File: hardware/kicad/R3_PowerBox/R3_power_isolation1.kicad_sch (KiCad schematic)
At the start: 13 parts, among them U3 RS3E-0505S/H3

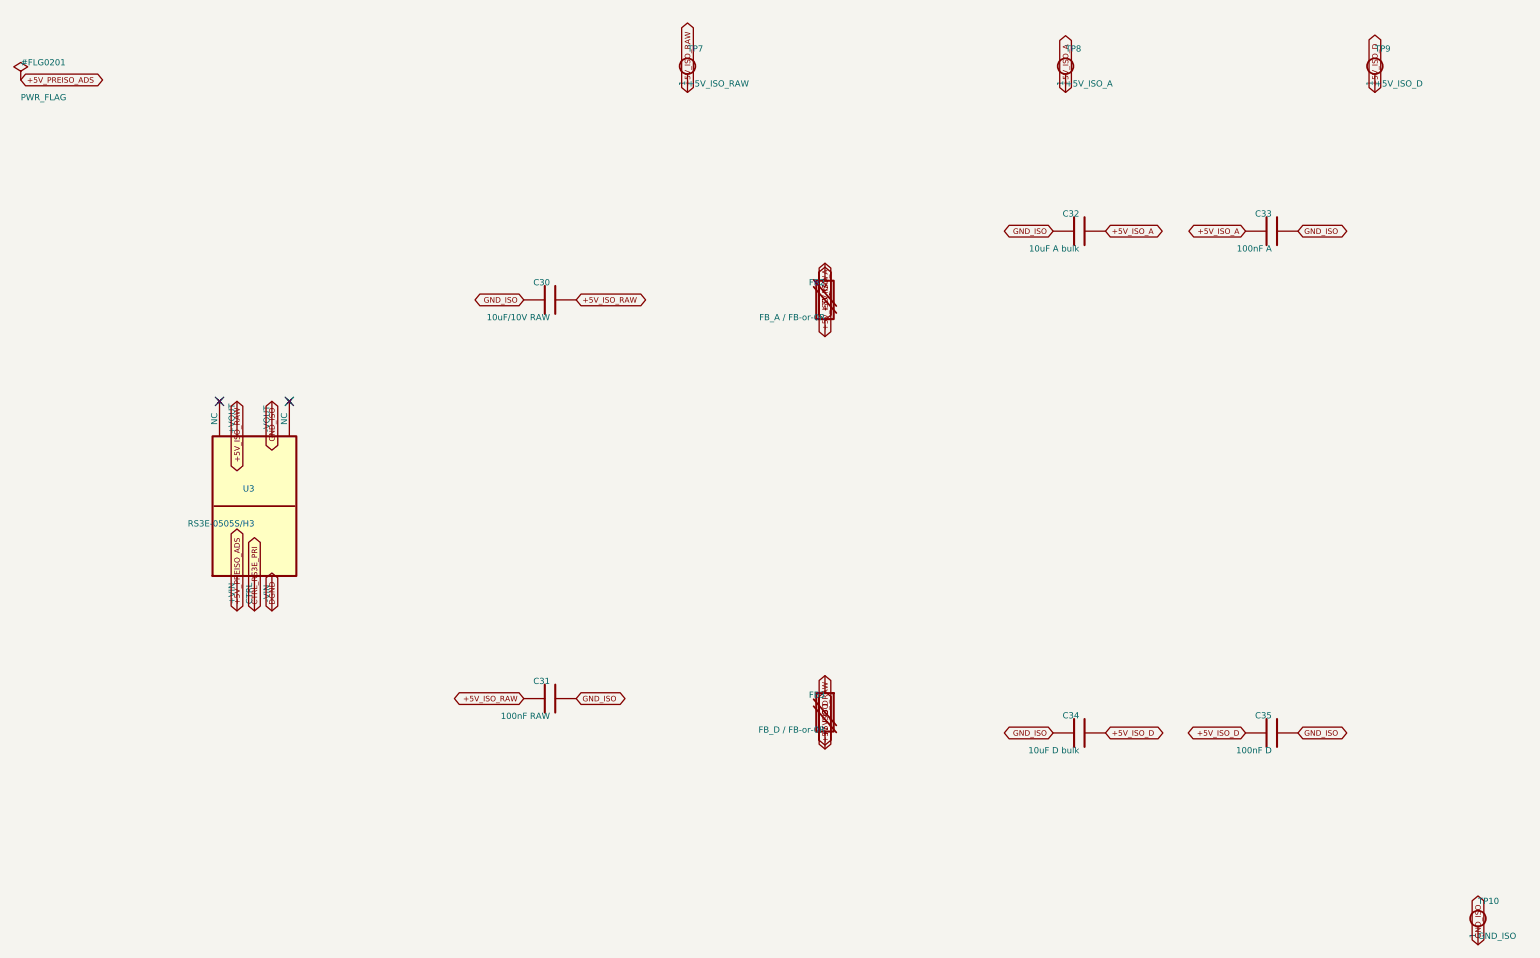
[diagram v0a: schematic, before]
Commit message: Rev.A review fixes: local charger power-stage reroute checkpoint
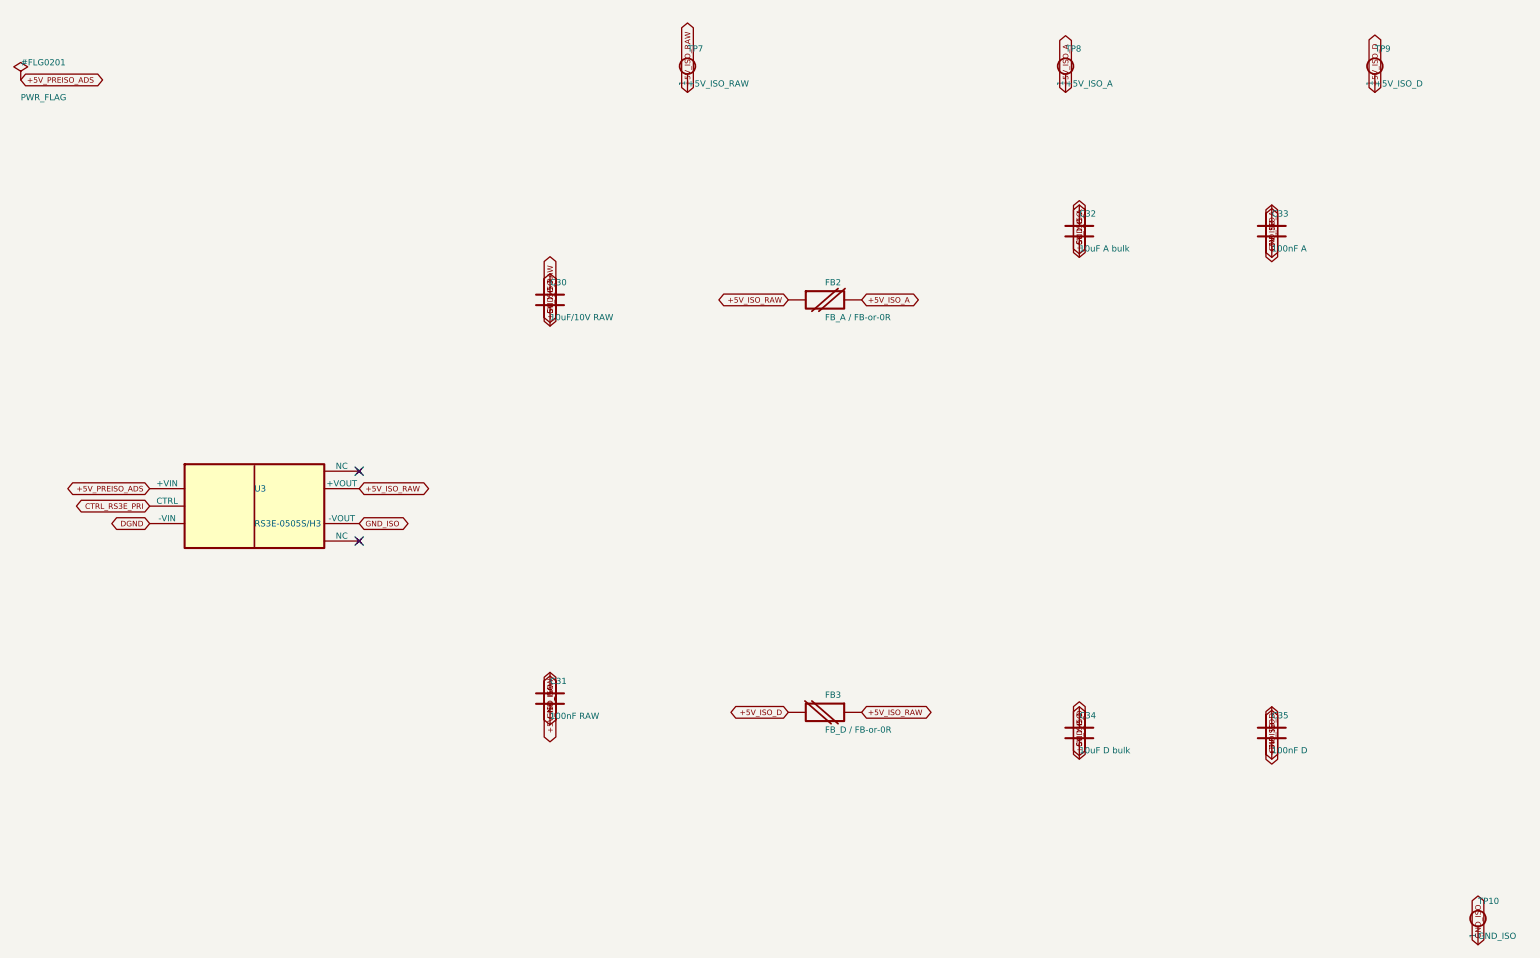
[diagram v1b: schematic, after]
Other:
- moved on the sheet: C30, C31, C32, C33, C34, C35, FB2, FB3, U3
